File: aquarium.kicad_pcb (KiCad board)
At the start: 2 copper layers, 104 x 47 mm, 40 parts, among them U1 MOC3063, U2 MOC3063

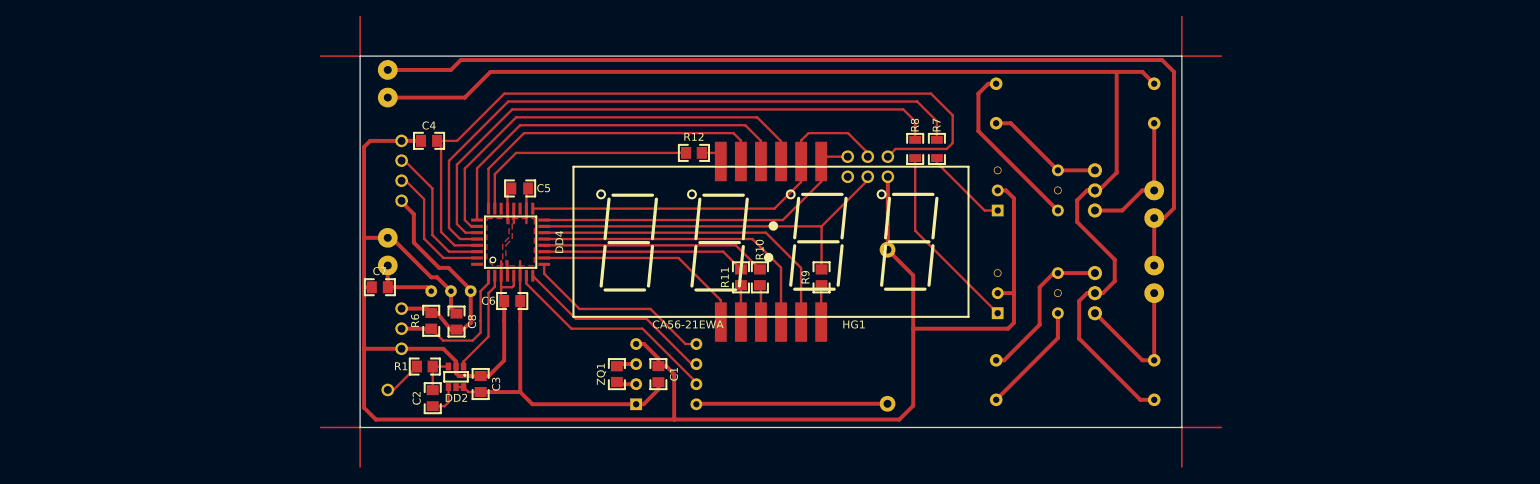
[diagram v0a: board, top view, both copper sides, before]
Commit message: New version of the controller (schematic and pcb).
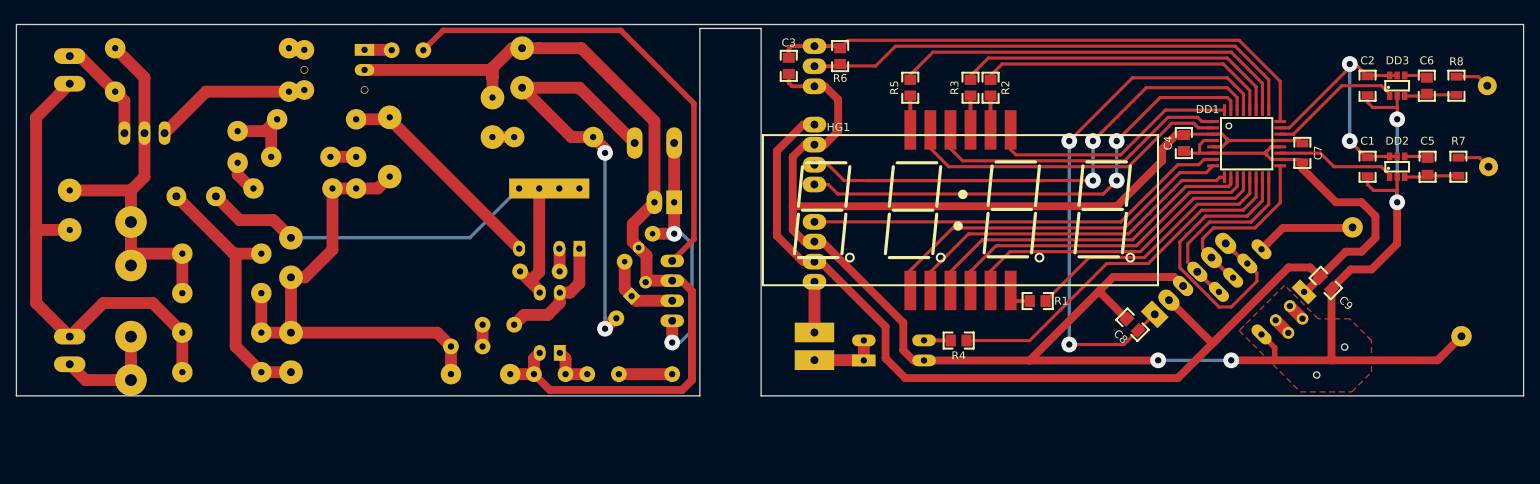
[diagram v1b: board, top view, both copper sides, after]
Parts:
- removed G***: LOGO, aquarium:logo
- removed VS2: BT137, Транзисторы:TO220
- added C10: 6.8мк, Конденсаторы:CPH_5_10x16mm, B.Cu at (84.2, 120.5)
- added C11: 22мк, Конденсаторы:CPH_5_13x25mm, B.Cu at (84.2, 108.5)
- added C12: 100н, Конденсаторы:C_5x3mm, B.Cu at (115.8, 110.2)
- added C13: 10н, Конденсаторы:C_7.5x4mm, B.Cu at (85.5, 95.8)
- added C14: 2н2, Конденсаторы:C_7.5x4mm, B.Cu at (108.2, 123.2)
- added C15: 1000мк, Конденсаторы:CPH_5_10x20mm, B.Cu at (113.5, 84.5)
- added C16: 100мк, Конденсаторы:CP_2.5x6mm, B.Cu at (131.5, 101.5)
- added C17: 47мк, Конденсаторы:CP_2.5x5mm, B.Cu at (128.2, 112.5)
- added C9: 0.1, Конденсаторы:SMD_0805, F.Cu at (215.2, 111.7)
- added DA2: 78L05, Транзисторы:TO92-250, B.Cu at (128.2, 107.2)
- added DD5: DS18B20, Разъемы:PLS-3, B.Cu at (150.5, 84.3)
- added FU1: 3.15A, Прочее:FU_5x20mm, B.Cu at (64.0, 114.0)
- added L1: 1мГн, Дроссели:Ind_5x8mm, B.Cu at (72.2, 100.8)
- added L2: 100мкГн, Дроссели:Ind_5x8mm, B.Cu at (130.2, 94.0)
- added R13: 1M8, Резисторы:RV_0.25, B.Cu at (110.5, 117.0)
- added R14: 1к, Резисторы:RV_0.25, B.Cu at (77.5, 94.5)
- added R15: 100, Резисторы:RV_0.25, B.Cu at (92.5, 97.8)
- added R16: 390, Резисторы:RV_0.25, B.Cu at (123.8, 123.2)
- added R17: 2к, Резисторы:RV_0.25, B.Cu at (117.0, 123.2)
- added RU1: 275B, Резисторы:FNR-05, B.Cu at (56.2, 102.5)
- added T1: E16, Трансформаторы:E16_5_10mm, B.Cu at (103.2, 93.2)
- added VD1: 1N4007, Диоды:DO-41, B.Cu at (75.5, 118.0)
- added VD2: 1N4007, Диоды:DO-41, B.Cu at (75.5, 123.0)
- added VD3: 1N4007, Диоды:DO-41, B.Cu at (75.5, 113.0)
- added VD4: 1N4007, Диоды:DO-41, B.Cu at (75.5, 108.0)
- added VD5: P6KE150A, Диоды:DO-15, B.Cu at (84.5, 99.8)
- added VD6: UF4007, Диоды:DO-41, B.Cu at (87.5, 91.0)
- added VD7: 1N5819, Диоды:DO-41, B.Cu at (117.5, 93.2)
- added VD8: 1N4741A, Диоды:DO-41, B.Cu at (129.0, 119.7)
- added VT1: IRLD014, Транзисторы:HVMDIP, B.Cu at (160.6, 120.2)
- added XP2: Sensor 2, Разъемы:PLS-1, B.Cu at (235.7, 86.8)
- added XT7: PLS-4, Разъемы:PLS-4, B.Cu at (132.5, 112.7)
- C2: value 2n2 -> 0.1
- C5, C6: value 0.1 -> 3n3
- DA1: value 78L05 -> TNY274; footprint Транзисторы:TO92-250 -> Микросхемы:PDIP-8C
- DD1: value DS18B20 -> ATMEGA8A; footprint Разъемы:PLS-3 -> Микросхемы:TQFP32-30; moved to F.Cu
- DD3: value DS1302 -> AT42QT1011; footprint Микросхемы:DIP8-300 -> Транзисторы:SOT23-6; moved to F.Cu
- DD4: value ATMEGA8A -> DS1302; footprint Микросхемы:TQFP32-30 -> Микросхемы:DIP8-300; moved to B.Cu
- GB1: value 3V -> 3В
- R1: value 100k -> 30
- R10, R9: value 30 -> 360; footprint Резисторы:R_0805 -> Резисторы:RH_2; moved to B.Cu
- R11: value 30 -> 620; footprint Резисторы:R_0805 -> Резисторы:RV_0.25; moved to B.Cu
- R12: value 30 -> 1M8; footprint Резисторы:R_0805 -> Резисторы:RV_0.25; moved to B.Cu
- R2, R3, R4, R5: value 360 -> 30; footprint Резисторы:RH_2 -> Резисторы:R_0805; moved to F.Cu
- R7, R8: value 620 -> 100k
- U2: value MOC3063 -> PC817A; footprint Микросхемы:DIP6-300 -> Микросхемы:DIP4-300
- XP1: value Sensor -> Sensor 1
- XT1, XT3: value DG350-3.5-02P-14 -> PLS-4; footprint Разъемы:DG-350-2 -> Разъемы:PLS-4
- XT2: value DG350-3.5-02P-14 -> PLS-6; footprint Разъемы:DG-350-2 -> Разъемы:PLS-6
- XT5: value PLS-4 -> DG350-3.5-02P-14; footprint Разъемы:PLS-4 -> Разъемы:DG-350-2
- XT6: value PLD-6 -> DG350-3.5-02P-14; footprint Разъемы:PLD-6 -> Разъемы:DG-350-2
- ZQ1: footprint Резисторы:R_0805 -> Прочее:HC_3.0x8.0mm; moved to B.Cu
- moved XP1 142.1 mm to (235.8, 97.0), turned to 0 degrees
- moved C2 124.7 mm to (220.5, 86.8)
- moved DD2 122.0 mm to (224.2, 97.0), turned to 0 degrees
- moved VS1 120.5 mm to (65.7, 92.8), turned to 0 degrees
- moved C6 118.9 mm to (228.0, 86.8), turned to 270 degrees
- moved C7 118.0 mm to (212.2, 95.2), turned to 270 degrees
- moved C5 114.9 mm to (228.1, 97.0), turned to 270 degrees
- moved DD1 109.5 mm to (205.2, 94.1), turned to 0 degrees
- moved XT2 104.5 mm to (198.1, 111.2), turned to 45 degrees
- moved XT6 101.7 mm to (56.2, 84.8), turned to 90 degrees
- moved DD3 99.4 mm to (224.2, 86.8), turned to 0 degrees
- moved C4 95.5 mm to (197.2, 94.0), turned to 270 degrees
- moved DD4 95.2 mm to (207.1, 112.8), turned to 225 degrees
- moved C1 93.5 mm to (220.5, 97.0), turned to 90 degrees
- moved U1 89.1 mm to (89.8, 84.8), turned to 270 degrees
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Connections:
- C1 pad 1: +5B -> /SENS_PWR
- C2 pad 1: Net-(C2-Pad1) -> /SENS_PWR
- C2 pad 2: Net-(C2-Pad2) -> GND
- C3 pad 1: +5B -> /TEMP_PWR
- C4 pad 1: /~RESET -> +5B
- C5 pad 1: +5B -> Net-(C5-Pad1)
- C5 pad 2: GND -> Net-(C5-Pad2)
- C6 pad 1: +5B -> Net-(C6-Pad1)
- C6 pad 2: GND -> Net-(C6-Pad2)
- C7 pad 1: Vin -> +5B
- C8 pad 1: +5B -> /~RESET
- DA1 pad 1: +5B -> Net-(DA1-Pad1)
- DA1 pad 2: GND -> Net-(C12-Pad1)
- DD1 pad 1: GND -> /F
- DD1 pad 2: /TEMP -> /A
- DD1 pad 3: +5B -> GND
- DD2 pad 1: /SENS -> /SENS_1
- DD2 pad 3: Net-(C2-Pad1) -> Net-(C5-Pad1)
- DD2 pad 4: Net-(C2-Pad2) -> Net-(C5-Pad2)
- DD2 pad 5: +5B -> /SENS_PWR
- DD2 pad 6: +5B -> /SENS_PWR
- DD3 pad 1: +5B -> /SENS_2
- DD3 pad 2: Net-(DD3-Pad2) -> GND
- DD3 pad 3: Net-(DD3-Pad3) -> Net-(C6-Pad1)
- DD3 pad 4: GND -> Net-(C6-Pad2)
- DD3 pad 5: /RTC_CE -> /SENS_PWR
- DD3 pad 6: /RTC_IO -> /SENS_PWR
- DD4 pad 1: /TEMP -> +5B
- DD4 pad 2: /SENS -> Net-(DD4-Pad2)
- DD4 pad 3: GND -> Net-(DD4-Pad3)
- DD4 pad 4: +5B -> GND
- DD4 pad 5: GND -> /MISO
- DD4 pad 6: +5B -> /RTC_IO
- DD4 pad 7: /RTC_SCLK -> /MOSI
- DD4 pad 8: /RTC_IO -> Net-(DD4-Pad8)
- GB1 pad 1: VBAT -> Net-(DD4-Pad8)
- R1 pad 1: Net-(R1-Pad1) -> /DGT4
- R1 pad 2: Net-(C2-Pad1) -> Net-(HG1-Pad6)
- R10 pad 1: /DGT2 -> Net-(R10-Pad1)
- R10 pad 2: Net-(HG1-Pad9) -> Net-(R10-Pad2)
- R11 pad 1: /DGT3 -> Net-(R11-Pad1)
- R11 pad 2: Net-(HG1-Pad8) -> Net-(R11-Pad2)
- R12 pad 1: /DGT4 -> Net-(C10-Pad1)
- R12 pad 2: Net-(HG1-Pad6) -> Net-(R12-Pad2)
- R2 pad 1: Net-(R2-Pad1) -> /DGT3
- R2 pad 2: Net-(R2-Pad2) -> Net-(HG1-Pad8)
- R3 pad 1: Net-(R3-Pad1) -> /DGT2
- R3 pad 2: Net-(R3-Pad2) -> Net-(HG1-Pad9)
- R4 pad 1: Net-(R4-Pad1) -> /LIGHT
- R4 pad 2: Net-(R2-Pad2) -> Net-(R4-Pad2)
- R5 pad 1: Net-(R5-Pad1) -> /DGT1
- R5 pad 2: Net-(R5-Pad2) -> Net-(HG1-Pad12)
- R6 pad 1: +5B -> /TEMP
- R6 pad 2: /TEMP -> /TEMP_PWR
- R7 pad 2: /HEAT -> Net-(C5-Pad1)
- R8 pad 2: /LIGHT -> Net-(C6-Pad1)
- R9 pad 1: /DGT1 -> Net-(R9-Pad1)
- R9 pad 2: Net-(HG1-Pad12) -> Net-(FU1-Pad2)
- U1 pad 1: Net-(R7-Pad1) -> Net-(R11-Pad1)
- U1 pad 4: Net-(R3-Pad1) -> Net-(R10-Pad1)
- U1 pad 6: Net-(R2-Pad1) -> Net-(R9-Pad1)
- U2 pad 1: Net-(R8-Pad1) -> Net-(R16-Pad2)
- U2 pad 3: (no net) -> Net-(C11-Pad2)
- U2 pad 4: Net-(R5-Pad1) -> Net-(DA1-Pad1)
- VS1 pad 1: Net-(R3-Pad2) -> Net-(R10-Pad2)
- VS1 pad 2: Net-(R2-Pad2) -> Net-(FU1-Pad2)
- VS1 pad 3: Net-(R3-Pad1) -> Net-(R10-Pad1)
- XP1 pad 1: Net-(R1-Pad1) -> Net-(R7-Pad1)
- XT1 pad 1: Vin -> +5B
- XT2 pad 1: Net-(R2-Pad2) -> /~RESET
- XT2 pad 2: Net-(XT2-Pad2) -> +5B
- XT3 pad 1: Net-(R3-Pad2) -> +12B
- XT3 pad 2: Net-(XT2-Pad2) -> +5B
- XT4 pad 1: Net-(R5-Pad2) -> +12B
- XT4 pad 2: Net-(XT2-Pad2) -> Net-(VT1-Pad1)
- XT5 pad 1: +5B -> Net-(FU1-Pad1)
- XT5 pad 2: /TX -> Net-(RU1-Pad1)
- XT6 pad 1: /E -> Net-(RU1-Pad1)
- XT6 pad 2: +5B -> Net-(R10-Pad2)
- ZQ1 pad 1: Net-(DD3-Pad3) -> Net-(DD4-Pad3)
- ZQ1 pad 2: Net-(DD3-Pad2) -> Net-(DD4-Pad2)
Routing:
- net Net-(R2-Pad2): track 153.4 -> 0.00 mm
- net GND: track 246.7 -> 395.8 mm, vias 0 -> 4
- net Net-(XT2-Pad2): track 126.9 -> 0.00 mm
- net +5B: track 83.9 -> 169.0 mm
- net /TEMP_PWR: track 0.00 -> 71.2 mm
- net /RX: track 17.8 -> 86.8 mm, vias 0 -> 2
- net Net-(C11-Pad2): track 0.00 -> 66.7 mm
- net Net-(C10-Pad1): track 0.00 -> 62.5 mm
- net Net-(RU1-Pad1): track 0.00 -> 62.3 mm
- net Net-(R11-Pad2): track 0.00 -> 60.2 mm
- net Net-(C15-Pad1): track 0.00 -> 55.6 mm, vias 0 -> 2
- net Net-(FU1-Pad2): track 0.00 -> 49.1 mm
- net /TX: track 16.5 -> 62.5 mm, vias 0 -> 2
- net /TEMP: track 18.6 -> 64.4 mm
- net +12B: track 0.00 -> 40.4 mm, vias 0 -> 2
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- removed copper zone on F.Cu, net +5B
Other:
- board size 104 x 47 mm -> 190.8 x 47 mm
- net class Default: trace_width 0.25 -> 0.4; via_dia 0.6 -> 2; via_drill 0.4 -> 0.8
- board text added: "+"
- board text added: "+12V"
- board text added: "-"
- board text added: "MISO"
- board text added: "MOSI"
- board text added: "PICkit2"
- board text added: "SCK"
- board text added: "VCC"
- board text added: "~RESET"
- board text removed: "1"
- board text removed: "ISP"
